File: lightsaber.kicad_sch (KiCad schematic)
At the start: 7 parts, among them SW1 SW_Push, SW3 POWER, U1 C3 Pico

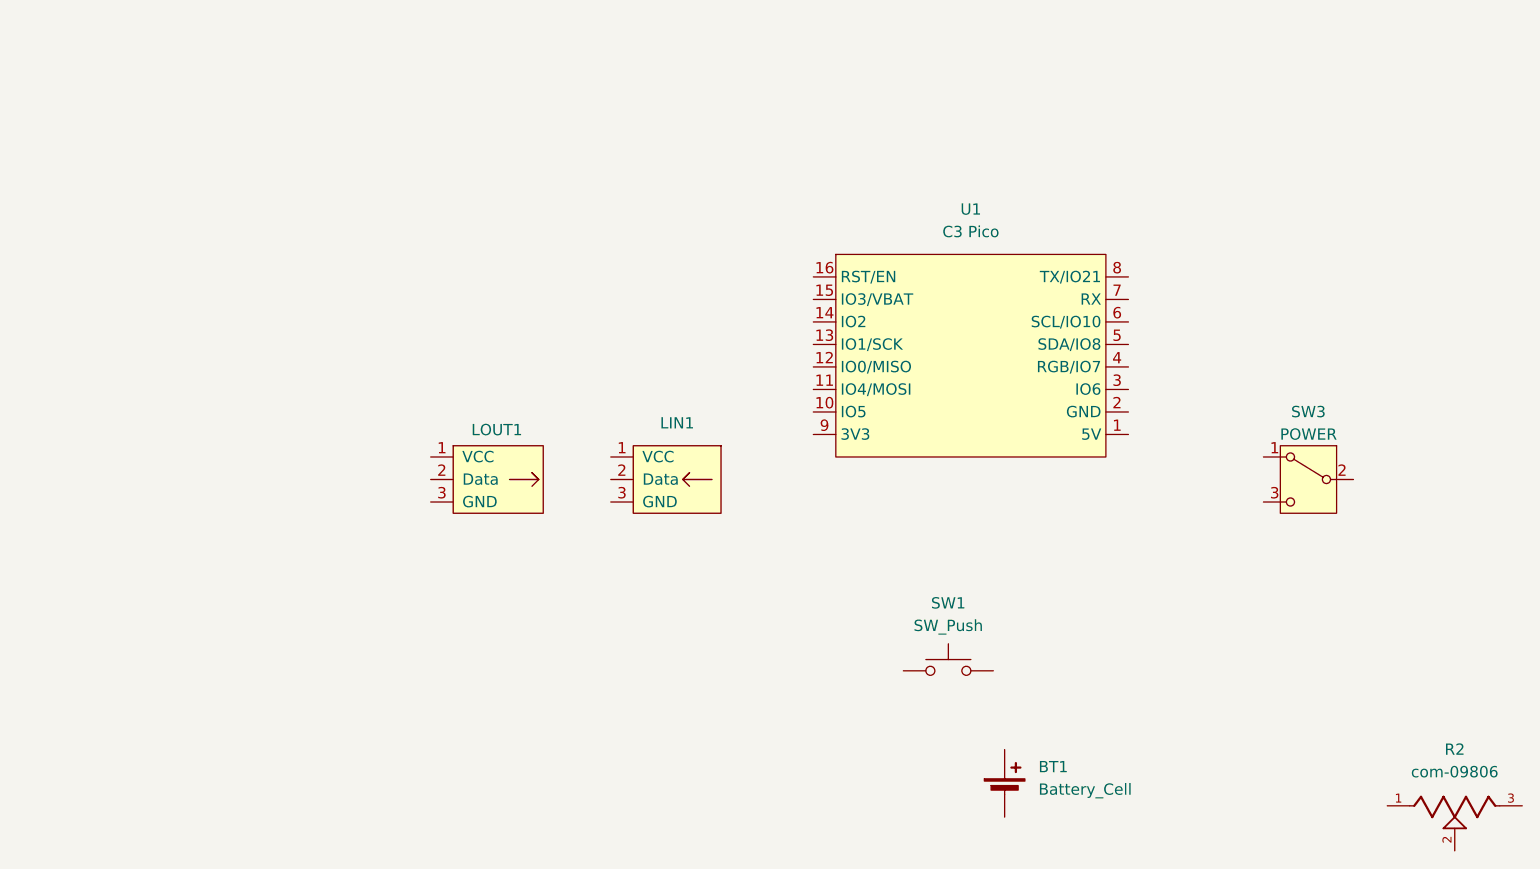
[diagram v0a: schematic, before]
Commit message: Preliminary PCB layout
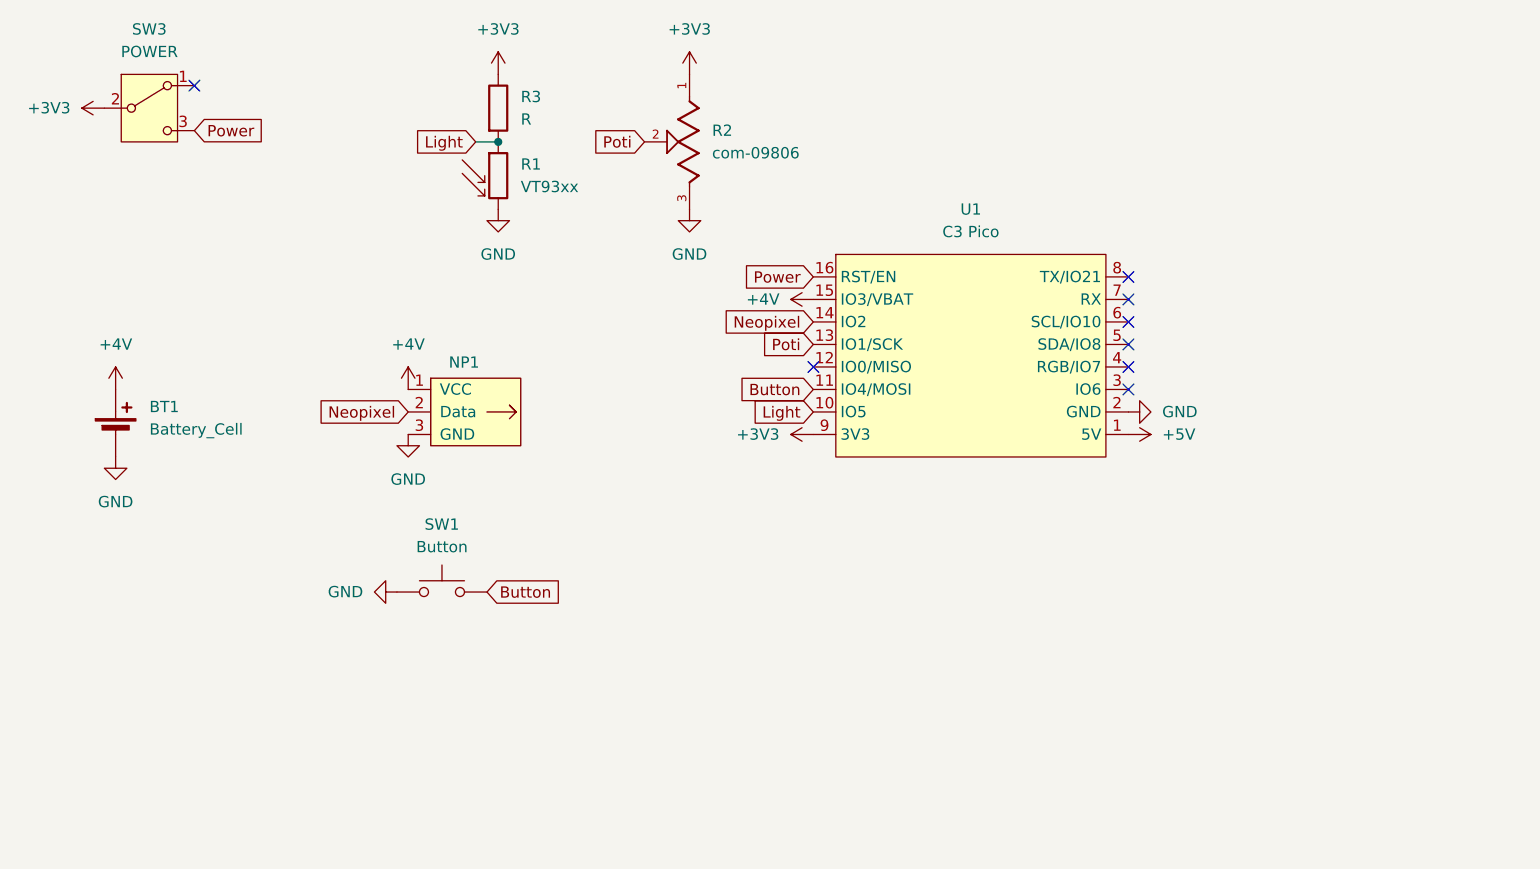
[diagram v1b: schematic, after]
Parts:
- removed LIN1: LEDs_In, neopixel-strip:neopixel-strip, symbol neopixel-strip:LEDs_In
- added R1: VT93xx, OptoDevice:R_LDR_4.9x4.2mm_P2.54mm_Vertical, symbol Sensor_Optical:VT93xx
- added R3: R, Resistor_SMD:R_0805_2012Metric_Pad1.20x1.40mm_HandSolder, symbol Device:R
- SW1: value SW_Push -> Button
- renumbered LOUT1 to NP1
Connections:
- net GND: now reaches SW1.1
- net GND: now also BT1.2 (-), NP1.3 (GND), R2.3, U1.2 (GND), R1.2
- net Button: now reaches SW1.2
- net Button: now also U1.11 (IO4/MOSI)
- net +5V: now reaches U1.1 (5V)
- net Light: now reaches U1.10 (IO5)
- net Light: now also R1.1, R3.2
- net Poti: now reaches U1.13 (IO1/SCK)
- net Poti: now also R2.2
- net Neopixel: now reaches U1.14 (IO2)
- net Neopixel: now also NP1.2 (Data)
- net +4V: now reaches U1.15 (IO3/VBAT)
- net +4V: now also BT1.1 (+), NP1.1 (VCC)
- net Power: now reaches U1.16 (RST/EN)
- net Power: now also SW3.3 (C)
- net +3V3: now reaches U1.9 (3V3)
- net +3V3: now also R2.1, SW3.2 (B), R3.1
- no-connect marks 0 -> 8
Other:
- moved on the sheet: BT1, NP1, R2, SW1, SW3
